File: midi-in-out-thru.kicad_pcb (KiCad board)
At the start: 2 copper layers, 72.6 x 48 mm, 19 parts, among them J1 uC, J2 IN, J3 OUT, J4 THRU, U1 74HC14, U2 H11L1

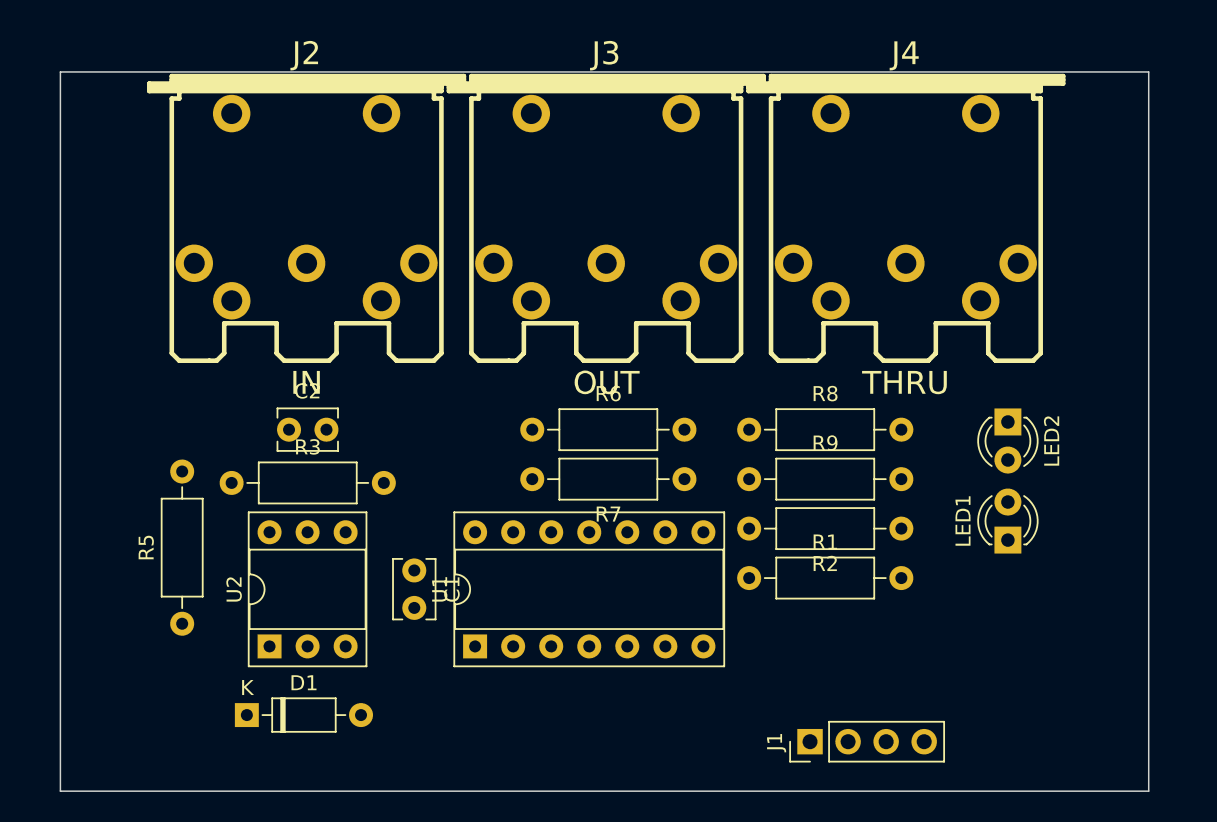
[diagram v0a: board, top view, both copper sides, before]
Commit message: Completed initial layout
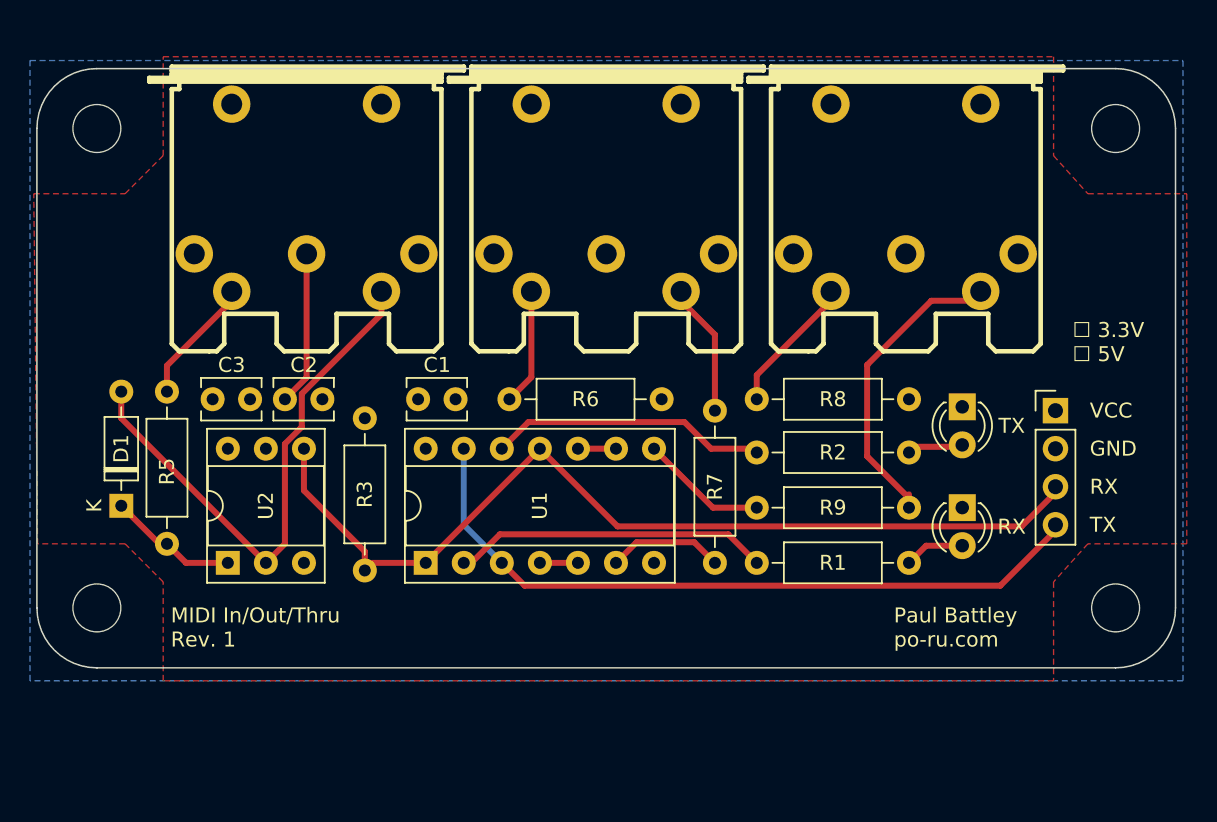
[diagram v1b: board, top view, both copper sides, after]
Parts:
- added C3: 100n, Capacitor_THT:C_Disc_D3.8mm_W2.6mm_P2.50mm, F.Cu at (93.7, 52.1)
- added H1: MountingHole, MountingHole:MountingHole_3.2mm_M3, F.Cu at (86.0, 34.0)
- added H2: MountingHole, MountingHole:MountingHole_3.2mm_M3, F.Cu at (154.0, 34.0)
- added H3: MountingHole, MountingHole:MountingHole_3.2mm_M3, F.Cu at (86.0, 66.0)
- added H4: MountingHole, MountingHole:MountingHole_3.2mm_M3, F.Cu at (154.0, 66.0)
- J2, J3, J4: footprint eurocad:MIDI_DIN5 -> Personal:MIDI_DIN5
- moved J1 27.5 mm to (150.0, 52.8), turned to 0 degrees
- moved D1 16.3 mm to (87.6, 59.2), turned to 90 degrees
- moved C1 11.4 mm to (107.4, 52.1), turned to 0 degrees
- moved R8 10.9 mm to (140.2, 52.1), turned to 180 degrees
- moved R1 10.7 mm to (140.2, 63.0), turned to 180 degrees
- moved R3 9.88 mm to (103.9, 53.3), turned to -90 degrees
- moved R6 8.87 mm to (123.7, 52.1), turned to 180 degrees
- moved U1 6.48 mm to (108.0, 63.0)
- moved U2 6.23 mm to (94.7, 63.0)
- moved R7 5.95 mm to (127.3, 63.0), turned to 90 degrees
- moved R5 5.43 mm to (90.7, 61.7)
- moved R2 5.11 mm to (140.2, 55.6)
- moved LED1 3.74 mm to (143.8, 59.3), turned to -90 degrees
- moved LED2 3.21 mm to (143.8, 52.6)
- moved C2 2.05 mm to (98.6, 52.1)
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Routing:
- net /RX: track 0.00 -> 62.7 mm
- net /TX: track 0.00 -> 48.2 mm
- net Net-(D1-Pad2): track 0.00 -> 36.7 mm
- net Net-(J4-Pad5): track 0.00 -> 21.2 mm
- net Net-(R1-Pad2): track 0.00 -> 21.1 mm
- net Net-(R2-Pad2): track 0.00 -> 18.6 mm
- net Net-(C2-Pad1): track 0.00 -> 10.3 mm
- net Net-(J4-Pad4): track 0.00 -> 9.25 mm
- net Net-(J3-Pad5): track 0.00 -> 8.90 mm
- net Net-(D1-Pad1): track 0.00 -> 8.69 mm
- net Net-(R9-Pad1): track 0.00 -> 8.49 mm
- net Net-(J2-Pad4): track 0.00 -> 8.48 mm
- net Net-(J3-Pad4): track 0.00 -> 7.81 mm
- net Net-(R7-Pad1): track 0.00 -> 7.75 mm
- net Net-(LED1-Pad2): track 0.00 -> 4.08 mm
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- added copper zone on F.Cu, net +3.3V
- added copper zone on B.Cu, net GND
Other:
- board size 72.6 x 48 mm -> 76 x 40 mm
- copper layers 2 -> 4
- board text added: "GND"
- board text added: "IN"
- board text added: "MIDI In/Out/Thru Rev. 1"
- board text added: "OUT"
- board text added: "Paul Battley po-ru.com"
- board text added: "RX"
- board text added: "THRU"
- board text added: "TX"
- board text added: "VCC"
- board text added: "☐ 3.3V ☐ 5V"
